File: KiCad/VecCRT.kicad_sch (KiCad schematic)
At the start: 77 parts, among them J1 RaspiGPIO, J2 K2, J3 Conn_01x03, J4 Conn_01x06, J5 Conn_01x03, J6 Conn_01x06, J7 K2, Q1 2N7000, Q10 2N7000, Q2 2N7002, Q3 2N7002, Q4 2N7000, Q5 2N7002, Q6 2N7002, Q9 2N7000, U1 MCP4822, U2 4066, U3 4066, U4 TL072, U5 TL072, U6 4011, U7 40106, U8 4011

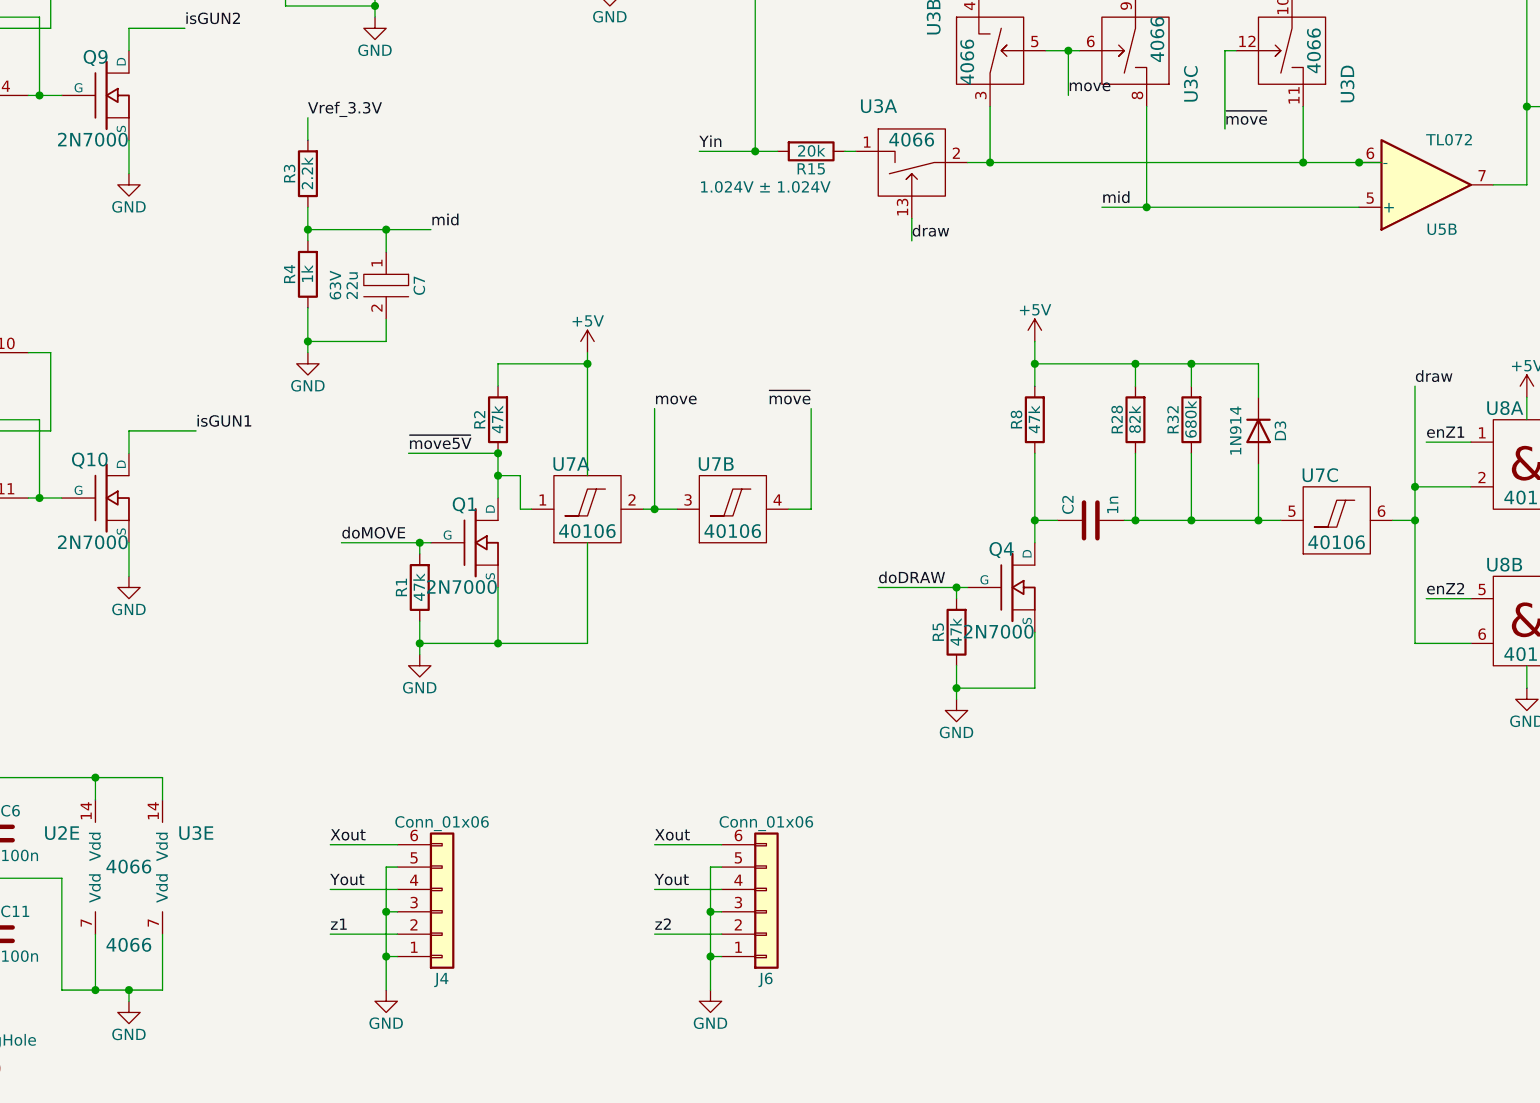
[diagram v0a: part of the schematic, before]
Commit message: minor changes
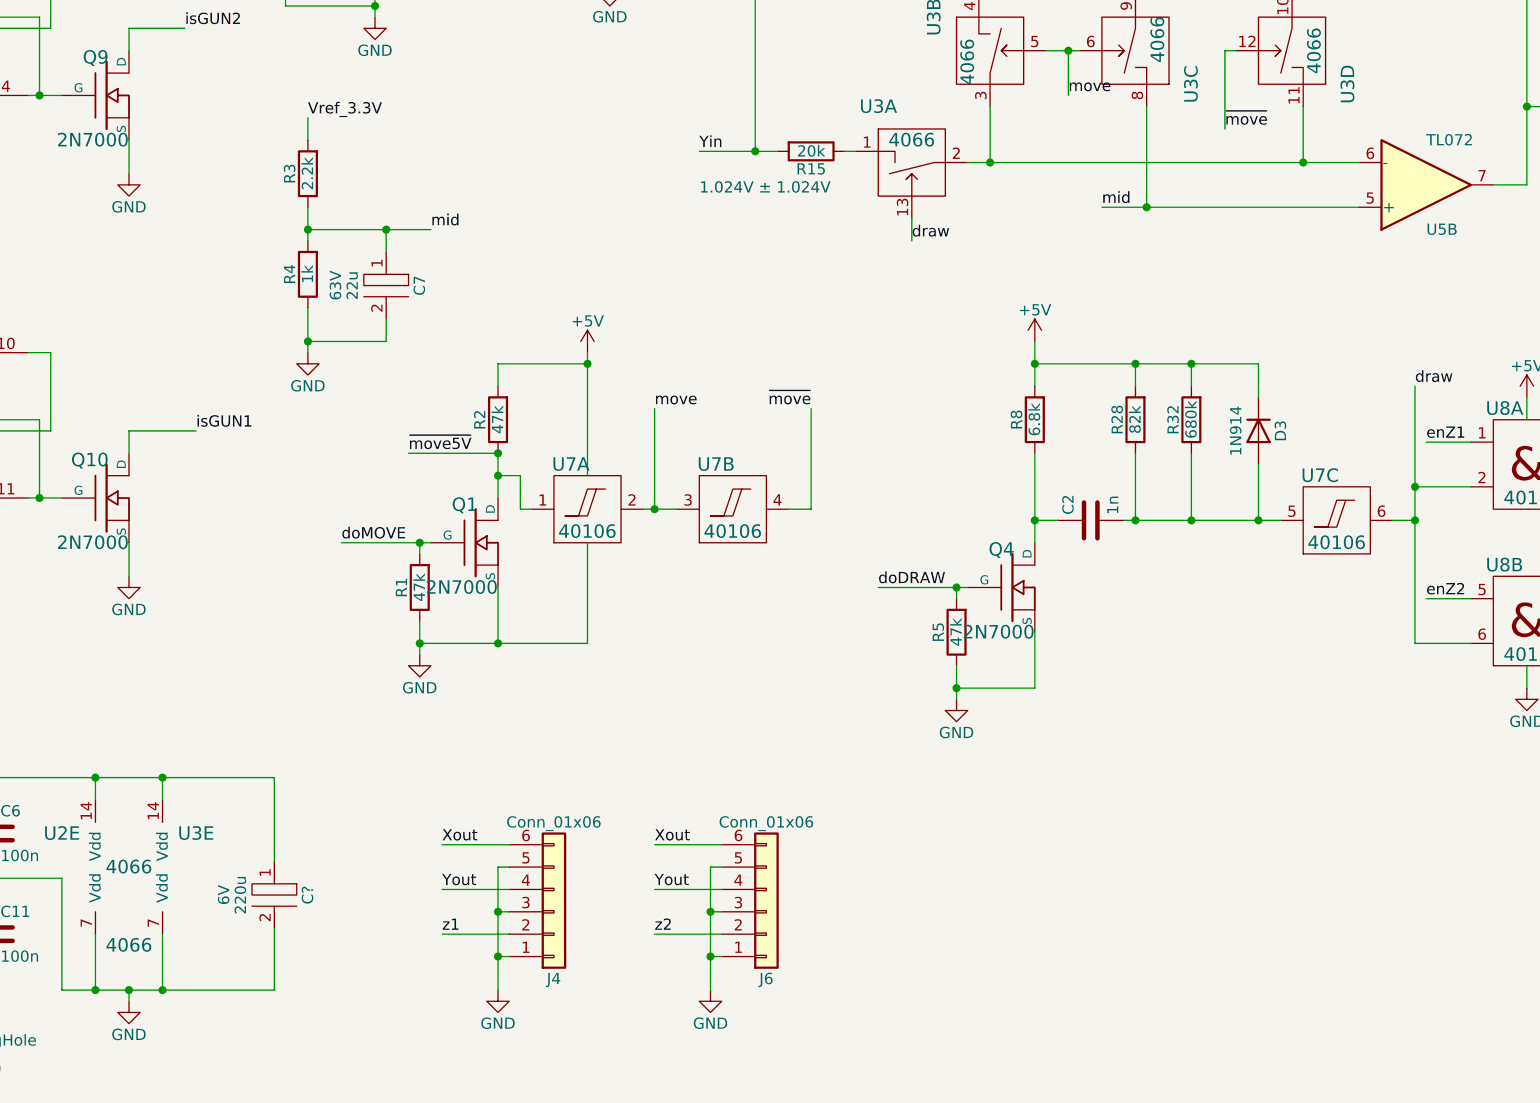
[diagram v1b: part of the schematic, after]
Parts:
- added C?: 220u, RG:C2-7, symbol rg:ELKO
- R8: value 47k -> 6.8k
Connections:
- net +5V: now also C?.1
- net GND: now also C?.2
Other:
- moved on the sheet: J4
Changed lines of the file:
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@@
   (junction (at 125.73 71.12) (diameter 0) (color 0 0 0 0)
   )
-  (junction (at 110.49 187.96) (diameter 0) (color 0 0 0 0)
+  (junction (at 123.19 187.96) (diameter 0) (color 0 0 0 0)
   )
   (junction (at 57.15 196.85) (diameter 0) (color 0 0 0 0)
@@
   (junction (at 114.3 146.05) (diameter 0) (color 0 0 0 0)
   )
-  (junction (at 110.49 193.04) (diameter 0) (color 0 0 0 0)
+  (junction (at 123.19 193.04) (diameter 0) (color 0 0 0 0)
   )
   (junction (at 251.46 137.16) (diameter 0) (color 0 0 0 0)
@@
   (junction (at 175.26 151.13) (diameter 0) (color 0 0 0 0)
   )
-  (junction (at 220.98 102.87) (diameter 0) (color 0 0 0 0)
-  )
   (junction (at 247.65 39.37) (diameter 0) (color 0 0 0 0)
   )
   (junction (at 38.1 124.46) (diameter 0) (color 0 0 0 0)
   )
+  (junction (at 85.09 196.85) (diameter 0) (color 0 0 0 0)
+  )
   (junction (at 177.8 69.85) (diameter 0) (color 0 0 0 0)
   )
@@
   (junction (at 251.46 154.94) (diameter 0) (color 0 0 0 0)
   )
+  (junction (at 85.09 172.72) (diameter 0) (color 0 0 0 0)
+  )
   (junction (at 135.89 81.28) (diameter 0) (color 0 0 0 0)
   )
@@
     (stroke (width 0.3048) (type default) (color 0 0 0 0))
   )
-  (wire (pts (xy 110.49 182.88) (xy 110.49 187.96))
+  (wire (pts (xy 123.19 182.88) (xy 123.19 187.96))
     (stroke (width 0.3048) (type default) (color 0 0 0 0))
   )
@@
     (stroke (width 0.3048) (type default) (color 0 0 0 0))
   )
-  (wire (pts (xy 220.98 102.87) (xy 223.52 102.87))
-    (stroke (width 0.3048) (type default) (color 0 0 0 0))
-  )
   (wire (pts (xy 196.85 96.52) (xy 196.85 107.95))
     (stroke (width 0.3048) (type default) (color 0 0 0 0))
@@
     (stroke (width 0.3048) (type default) (color 0 0 0 0))
   )
-  (wire (pts (xy 104.14 180.34) (xy 111.76 180.34))
+  (wire (pts (xy 116.84 180.34) (xy 124.46 180.34))
     (stroke (width 0.3048) (type default) (color 0 0 0 0))
   )
@@
     (stroke (width 0.3048) (type default) (color 0 0 0 0))
   )
-  (wire (pts (xy 110.49 193.04) (xy 111.76 193.04))
+  (wire (pts (xy 123.19 193.04) (xy 124.46 193.04))
     (stroke (width 0.3048) (type default) (color 0 0 0 0))
   )
@@
     (stroke (width 0.3048) (type default) (color 0 0 0 0))
   )
-  (wire (pts (xy 111.76 185.42) (xy 104.14 185.42))
+  (wire (pts (xy 124.46 185.42) (xy 116.84 185.42))
     (stroke (width 0.3048) (type default) (color 0 0 0 0))
   )
@@
     (stroke (width 0.3048) (type default) (color 0 0 0 0))
   )
+  (wire (pts (xy 97.79 182.245) (xy 97.79 172.72))
+    (stroke (width 0) (type default) (color 0 0 0 0))
+  )
   (wire (pts (xy 234.95 22.86) (xy 240.03 22.86))
     (stroke (width 0.3048) (type default) (color 0 0 0 0))
@@
     (stroke (width 0.3048) (type default) (color 0 0 0 0))
   )
+  (wire (pts (xy 97.79 196.85) (xy 85.09 196.85))
+    (stroke (width 0) (type default) (color 0 0 0 0))
+  )
   (wire (pts (xy 196.85 22.86) (xy 213.36 22.86))
     (stroke (width 0.3048) (type default) (color 0 0 0 0))
@@
     (stroke (width 0.3048) (type default) (color 0 0 0 0))
   )
-  (wire (pts (xy 110.49 196.85) (xy 110.49 193.04))
+  (wire (pts (xy 123.19 196.85) (xy 123.19 193.04))
     (stroke (width 0.3048) (type default) (color 0 0 0 0))
   )
@@
     (stroke (width 0.3048) (type default) (color 0 0 0 0))
   )
-  (wire (pts (xy 104.14 190.5) (xy 111.76 190.5))
+  (wire (pts (xy 116.84 190.5) (xy 124.46 190.5))
     (stroke (width 0.3048) (type default) (color 0 0 0 0))
   )
@@
     (stroke (width 0.3048) (type default) (color 0 0 0 0))
   )
+  (wire (pts (xy 97.79 172.72) (xy 85.09 172.72))
+    (stroke (width 0) (type default) (color 0 0 0 0))
+  )
   (wire (pts (xy 53.34 86.36) (xy 71.12 86.36))
     (stroke (width 0.3048) (type default) (color 0 0 0 0))
   )
-  (wire (pts (xy 111.76 182.88) (xy 110.49 182.88))
+  (wire (pts (xy 124.46 182.88) (xy 123.19 182.88))
     (stroke (width 0.3048) (type default) (color 0 0 0 0))
   )
@@
     (stroke (width 0.3048) (type default) (color 0 0 0 0))
   )
+  (wire (pts (xy 97.79 189.865) (xy 97.79 196.85))
+    (stroke (width 0) (type default) (color 0 0 0 0))
+  )
   (wire (pts (xy 33.02 64.77) (xy 33.02 62.23))
     (stroke (width 0.3048) (type default) (color 0 0 0 0))
@@
     (stroke (width 0.3048) (type default) (color 0 0 0 0))
   )
-  (wire (pts (xy 110.49 187.96) (xy 111.76 187.96))
+  (wire (pts (xy 123.19 187.96) (xy 124.46 187.96))
     (stroke (width 0.3048) (type default) (color 0 0 0 0))
   )
@@
     (stroke (width 0) (type default) (color 0 0 0 0))
   )
-  (wire (pts (xy 110.49 193.04) (xy 110.49 187.96))
+  (wire (pts (xy 123.19 193.04) (xy 123.19 187.96))
     (stroke (width 0.3048) (type default) (color 0 0 0 0))
   )
@@
     (effects (font (size 1.27 1.27)) (justify left bottom))
   )
-  (label "Yout" (at 104.14 185.42 0)
+  (label "Yout" (at 116.84 185.42 0)
     (effects (font (size 1.27 1.27)) (justify left bottom))
   )
@@
     (effects (font (size 1.27 1.27)) (justify left bottom))
   )
-  (label "z1" (at 104.14 190.5 0)
+  (label "z1" (at 116.84 190.5 0)
     (effects (font (size 1.27 1.27)) (justify left bottom))
   )
@@
     (effects (font (size 1.27 1.27)) (justify left bottom))
   )
-  (label "Xout" (at 104.14 180.34 0)
+  (label "Xout" (at 116.84 180.34 0)
     (effects (font (size 1.27 1.27)) (justify left bottom))
   )
@@
     (pin "1")
   )
-  (symbol (lib_id "Connector_Generic:Conn_01x06") (at 116.84 187.96 0) (mirror x) (unit 1)
+  (symbol (lib_id "Connector_Generic:Conn_01x06") (at 129.54 187.96 0) (mirror x) (unit 1)
     (in_bom yes) (on_board yes)
-    (property "Reference" "J4" (id 0) (at 116.84 195.58 0))
-    (property "Value" "Conn_01x06" (id 1) (at 116.84 177.8 0))
-    (property "Footprint" "RG:PSS_6" (id 2) (at 116.84 187.96 0)
+    (property "Reference" "J4" (id 0) (at 129.54 195.58 0))
+    (property "Value" "Conn_01x06" (id 1) (at 129.54 177.8 0))
+    (property "Footprint" "RG:PSS_6" (id 2) (at 129.54 187.96 0)
       (effects (font (size 1.27 1.27)) hide)
     )
-    (property "Datasheet" "~" (id 3) (at 116.84 187.96 0)
+    (property "Datasheet" "~" (id 3) (at 129.54 187.96 0)
       (effects (font (size 1.27 1.27)) hide)
     )
@@
     (in_bom yes) (on_board yes)
     (property "Reference" "R8" (id 0) (at 182.118 132.08 90))
-    (property "Value" "47k" (id 1) (at 184.15 132.08 90))
+    (property "Value" "6.8k" (id 1) (at 184.15 132.08 90))
     (property "Footprint" "RG:R4-2" (id 2) (at 185.928 132.08 90)
       (effects (font (size 1.27 1.27)) hide)
@@
     (pin "3")
   )
-  (symbol (lib_id "power:GND") (at 110.49 196.85 0) (unit 1)
+  (symbol (lib_id "power:GND") (at 123.19 196.85 0) (unit 1)
     (in_bom yes) (on_board yes)
-    (property "Reference" "#PWR025" (id 0) (at 110.49 203.2 0)
+    (property "Reference" "#PWR025" (id 0) (at 123.19 203.2 0)
       (effects (font (size 1.27 1.27)) hide)
     )
-    (property "Value" "GND" (id 1) (at 110.49 200.66 0))
-    (property "Footprint" "" (id 2) (at 110.49 196.85 0)
+    (property "Value" "GND" (id 1) (at 123.19 200.66 0))
+    (property "Footprint" "" (id 2) (at 123.19 196.85 0)
       (effects (font (size 1.27 1.27)) hide)
     )
-    (property "Datasheet" "" (id 3) (at 110.49 196.85 0)
+    (property "Datasheet" "" (id 3) (at 123.19 196.85 0)
       (effects (font (size 1.27 1.27)) hide)
     )
@@
     (pin "2")
   )
+  (symbol (lib_id "rg:ELKO") (at 97.79 187.325 270) (unit 1)
+    (in_bom yes) (on_board yes)
+    (property "Reference" "C?" (id 0) (at 101.6 186.055 0))
+    (property "Value" "220u" (id 1) (at 93.98 186.055 0))
+    (property "Footprint" "RG:C2-7" (id 2) (at 97.79 187.325 0)
+      (effects (font (size 1.524 1.524)) hide)
+    )
+    (property "Datasheet" "" (id 3) (at 97.79 187.325 0)
+      (effects (font (size 1.524 1.524)))
+    )
+    (property "Voltage" "6V" (id 4) (at 92.075 186.055 0))
+    (pin "1")
+    (pin "2")
+  )
   (symbol (lib_id "power:GND") (at 60.96 102.87 0) (unit 1)
     (in_bom yes) (on_board yes)
@@
       (reference "C11") (unit 1) (value "100n") (footprint "RG:SM-1206B")
     )
+    (path "/1ca25c26-93d8-469d-96b3-7b05369ae2a4"
+      (reference "C?") (unit 1) (value "220u") (footprint "RG:C2-7")
+    )
     (path "/00000000-0000-0000-0000-0000648bedcb"
       (reference "D1") (unit 1) (value "1N914") (footprint "Diode_THT:D_DO-35_SOD27_P7.62mm_Horizontal")
@@
     )
     (path "/00000000-0000-0000-0000-000064830a2d"
-      (reference "R8") (unit 1) (value "47k") (footprint "RG:R4-2")
+      (reference "R8") (unit 1) (value "6.8k") (footprint "RG:R4-2")
     )
     (path "/00000000-0000-0000-0000-00006453444b"
